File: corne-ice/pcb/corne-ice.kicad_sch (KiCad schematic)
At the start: 103 parts, among them SW1 SW_PUSH, SW2 SW_PUSH, SW22 SW_PUSH, SW23 SW_PUSH, SW24 SW_PUSH, SW25 SW_PUSH, SW26 SW_PUSH, SW27 SW_PUSH, SW28 SW_PUSH, SW29 SW_PUSH, SW3 SW_PUSH, SW30 SW_PUSH, SW31 SW_PUSH, SW32 SW_PUSH, SW33 SW_PUSH, SW34 SW_PUSH, SW35 SW_PUSH, SW36 SW_PUSH, SW37 SW_PUSH, SW38 SW_PUSH, SW39 SW_PUSH, SW4 SW_PUSH, SW40 SW_PUSH, SW41 SW_PUSH, SW42 SW_PUSH, SW43 RotaryEncoder_Switch, SW45 SW_PUSH, SW46 SW_PUSH, SW47 SW_PUSH, SW48 SW_PUSH, SW49 SW_PUSH, SW5 SW_PUSH, SW50 SW_PUSH, SW51 SW_PUSH, SW52 SW_PUSH, SW53 SW_PUSH, SW54 SW_PUSH, SW55 SW_PUSH, SW56 SW_PUSH, SW57 SW_PUSH, SW58 SW_PUSH, SW59 SW_PUSH, SW6 SW_PUSH, SW60 SW_PUSH, SW61 SW_PUSH, SW7 RotaryEncoder_Switch, U1 nice!nano, U2 nice!nano

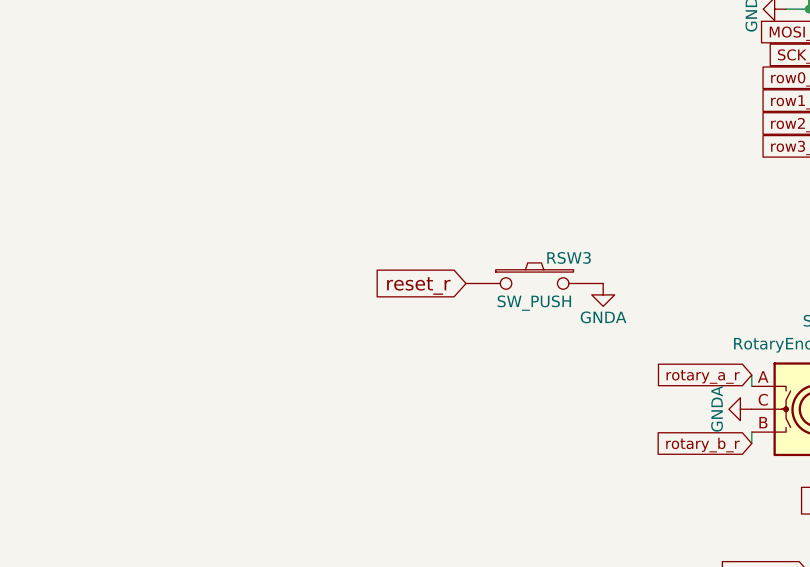
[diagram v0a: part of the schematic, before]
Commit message: Backup.
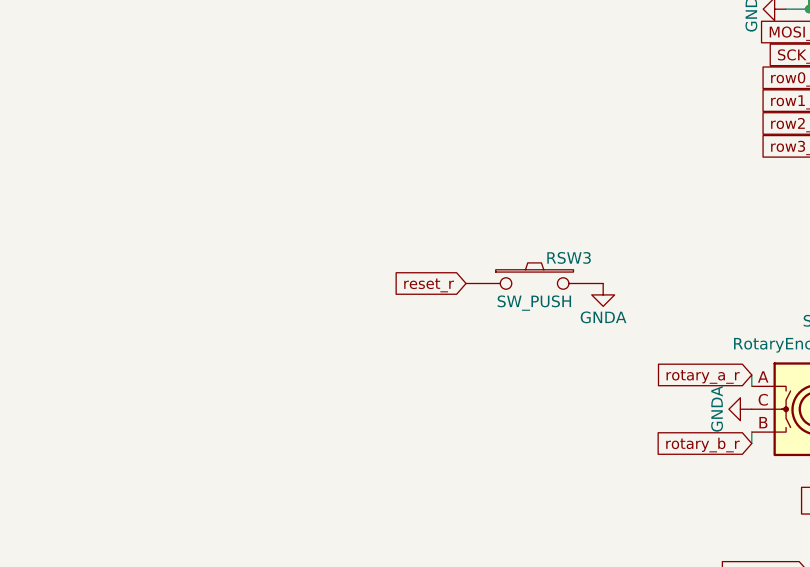
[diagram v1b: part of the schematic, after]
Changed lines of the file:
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@@
-    )
-  )
-  (global_label "reset_r" (shape input) (at 69.85 138.43 180) (fields_autoplaced)
-    (effects (font (size 1.524 1.524)) (justify right))
-    (property "Intersheetrefs" "${INTERSHEET_REFS}" (at 59.2881 138.43 0)
-      (effects (font (size 1.27 1.27)) (justify right) hide)
     )
   )
@@
       (effects (font (size 1.27 1.27)) (justify right) hide)
     )
+  )
+  (global_label "reset_r" (shape input) (at 69.85 138.43 180) (fields_autoplaced)
+    (effects (font (size 1.1938 1.1938)) (justify right))
+    (property "Intersheetrefs" "${INTERSHEET_REFS}" (at 61.5763 138.43 0)
+      (effects (font (size 1.27 1.27)) (justify right) hide)
+    )
